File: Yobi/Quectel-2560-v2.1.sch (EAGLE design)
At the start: 110 parts, among them IC1 LM2576S, IC2 LM2576S, J1 U.FL, T1 NPN, T2 PNP, T3 NPN, U1 ATMEGA1280AU, U2 Quectel M95, U3 QUECTEL-L80

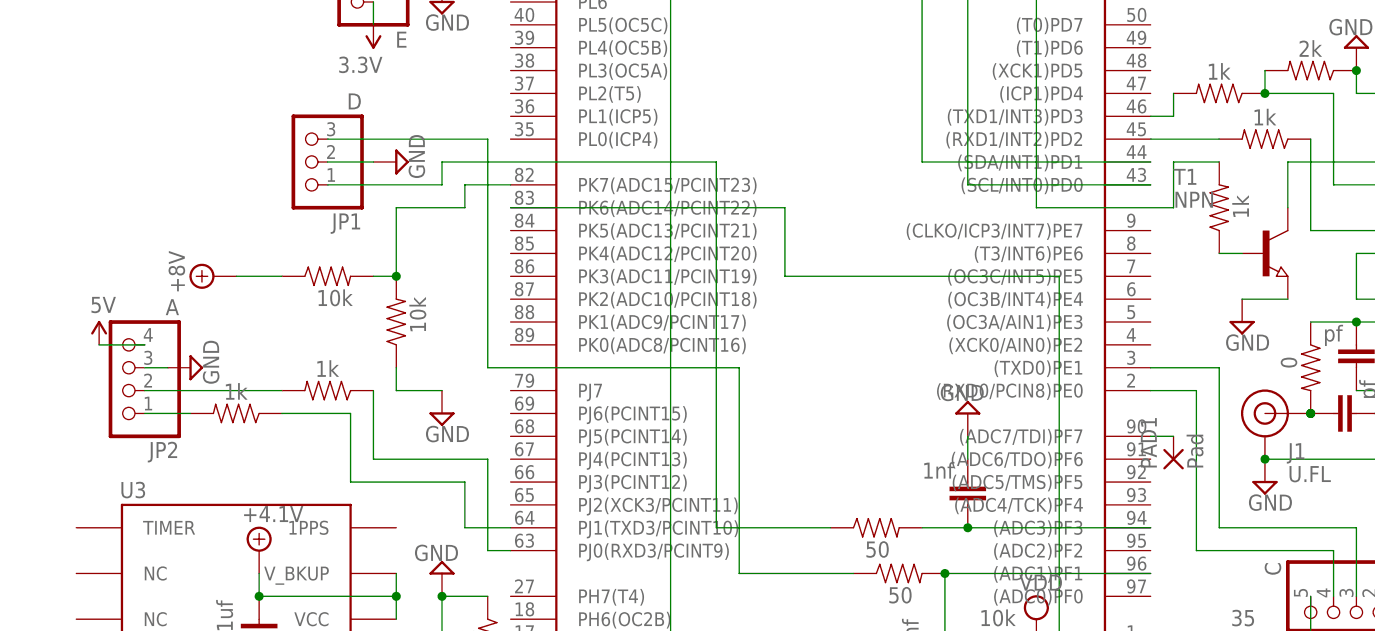
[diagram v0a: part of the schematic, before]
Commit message: cbdg
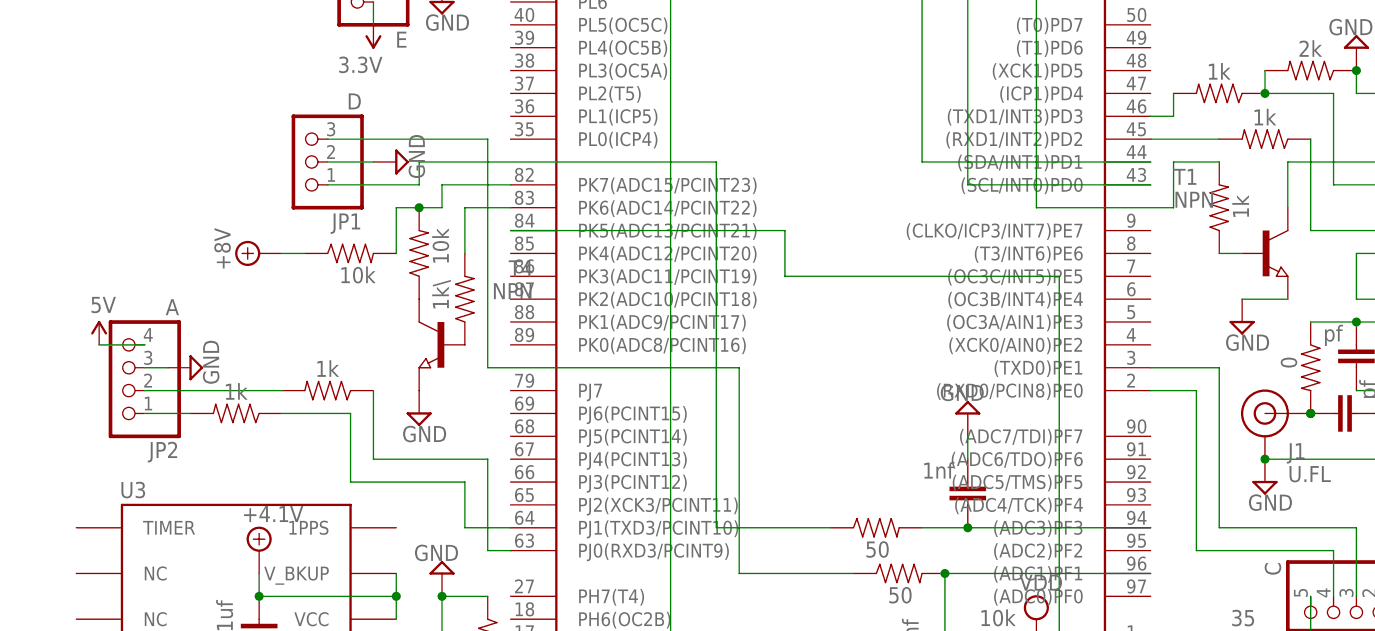
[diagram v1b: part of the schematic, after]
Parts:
- removed PAD1: Pad, wirepad:SMD2
- added R48: 1k\, SparkFun-Resistors:RESISTOR0805-RES
- added T4: NPN, semicon-smd-ipc:NPN-TRANSISTOR_SOT23
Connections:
- removed net N$69: PAD1.P, U1.(ADC7/TDI)PF7
- new net N$79: R44.1, T4.C
- new net N$80: R48.1, T4.B
- new net N$81: R48.2, U1.PK6(ADC14/PCINT22)
- net GND: now also T4.E; no longer R44.1
- net N$75: now also U1.PK5(ADC13/PCINT21); no longer U1.PK6(ADC14/PCINT22)
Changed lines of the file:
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@@
 <part name="DC16" library="resistor" deviceset="C-EU" device="C0805" value="0.1uf"/>
 <part name="JP11" library="pinhead" deviceset="PINHD-1X1" device="" value="Pogo Pin"/>
-<part name="PAD1" library="wirepad" deviceset="SMD2" device="" value="Pad"/>
 <part name="L4" library="rcl" deviceset="L-US" device="PIS2816" value="100uh"/>
 <part name="L2" library="rcl" deviceset="L-US" device="PIS2816" value="100uf"/>
+<part name="T4" library="semicon-smd-ipc" deviceset="NPN-TRANSISTOR_" device="SOT23" value="NPN"/>
+<part name="R48" library="SparkFun-Resistors" deviceset="RESISTOR" device="0805-RES" value="1k\"/>
 </parts>
 <sheets>
@@
 </instance>
 <instance part="SUPPLY54" gate="GND" x="104.14" y="71.12" rot="R270"/>
-<instance part="R43" gate="G$1" x="48.26" y="114.3" smashed="yes">
-<attribute name="VALUE" x="46.99" y="110.998" size="1.778" layer="96"/>
-</instance>
-<instance part="R44" gate="G$1" x="55.88" y="109.22" smashed="yes" rot="R90">
-<attribute name="VALUE" x="59.182" y="107.95" size="1.778" layer="96" rot="R90"/>
-</instance>
-<instance part="SUPPLY55" gate="+8V" x="35.56" y="114.3" rot="R90"/>
-<instance part="SUPPLY58" gate="GND" x="60.96" y="99.06"/>
+<instance part="R43" gate="G$1" x="50.8" y="116.84" smashed="yes">
+<attribute name="VALUE" x="49.53" y="113.538" size="1.778" layer="96"/>
+</instance>
+<instance part="R44" gate="G$1" x="58.42" y="116.84" smashed="yes" rot="R90">
+<attribute name="VALUE" x="61.722" y="115.57" size="1.778" layer="96" rot="R90"/>
+</instance>
+<instance part="SUPPLY55" gate="+8V" x="40.64" y="116.84" rot="R90"/>
+<instance part="SUPPLY58" gate="GND" x="58.42" y="99.06"/>
 <instance part="IC2" gate="A" x="142.24" y="292.1"/>
 <instance part="SUPPLY63" gate="+8V" x="119.38" y="297.18" rot="R90"/>
@@
 </instance>
 <instance part="JP11" gate="G$1" x="187.96" y="292.1"/>
-<instance part="PAD1" gate="1" x="142.24" y="93.98" rot="R90"/>
 <instance part="L4" gate="G$1" x="101.6" y="274.32" rot="R90"/>
 <instance part="L2" gate="G$1" x="165.1" y="292.1" rot="R90"/>
+<instance part="T4" gate="G$1" x="60.96" y="106.68" rot="MR0"/>
+<instance part="R48" gate="G$1" x="63.5" y="111.76" smashed="yes" rot="R90">
+<attribute name="VALUE" x="61.722" y="110.49" size="1.778" layer="96" rot="R90"/>
+</instance>
 </instances>
 <busses>
@@
 </segment>
 <segment>
+<pinref part="T4" gate="G$1" pin="E"/>
 <pinref part="SUPPLY58" gate="GND" pin="GND"/>
-<pinref part="R44" gate="G$1" pin="1"/>
-<wire x1="55.88" y1="104.14" x2="55.88" y2="101.6" width="0.1524" layer="91"/>
-<wire x1="55.88" y1="101.6" x2="60.96" y2="101.6" width="0.1524" layer="91"/>
 </segment>
 </net>
@@
 <segment>
 <pinref part="SUPPLY55" gate="+8V" pin="+8V"/>
-<wire x1="38.1" y1="114.3" x2="43.18" y2="114.3" width="0.1524" layer="91"/>
+<wire x1="43.18" y1="116.84" x2="45.72" y2="116.84" width="0.1524" layer="91"/>
 <pinref part="R43" gate="G$1" pin="1"/>
 </segment>
@@
 <wire x1="91.44" y1="86.36" x2="104.14" y2="86.36" width="0.1524" layer="91"/>
 <pinref part="R21" gate="G$1" pin="1"/>
-<wire x1="91.44" y1="127" x2="60.96" y2="127" width="0.1524" layer="91"/>
+<wire x1="91.44" y1="127" x2="58.42" y2="127" width="0.1524" layer="91"/>
 <pinref part="JP1" gate="A" pin="1"/>
-<wire x1="60.96" y1="127" x2="60.96" y2="124.46" width="0.1524" layer="91"/>
-<wire x1="60.96" y1="124.46" x2="48.26" y2="124.46" width="0.1524" layer="91"/>
+<wire x1="58.42" y1="127" x2="58.42" y2="124.46" width="0.1524" layer="91"/>
+<wire x1="58.42" y1="124.46" x2="48.26" y2="124.46" width="0.1524" layer="91"/>
 </segment>
 </net>
@@
 <wire x1="129.54" y1="71.12" x2="129.54" y2="114.3" width="0.1524" layer="91"/>
 <wire x1="129.54" y1="114.3" x2="99.06" y2="114.3" width="0.1524" layer="91"/>
-<pinref part="U1" gate="1" pin="PK6(ADC14/PCINT22)"/>
-<wire x1="99.06" y1="114.3" x2="99.06" y2="121.92" width="0.1524" layer="91"/>
-<wire x1="99.06" y1="121.92" x2="68.58" y2="121.92" width="0.1524" layer="91"/>
+<wire x1="99.06" y1="114.3" x2="99.06" y2="119.38" width="0.1524" layer="91"/>
+<pinref part="U1" gate="1" pin="PK5(ADC13/PCINT21)"/>
+<wire x1="68.58" y1="119.38" x2="99.06" y2="119.38" width="0.1524" layer="91"/>
 </segment>
 </net>
 <net name="N$76" class="0">
 <segment>
+<pinref part="R44" gate="G$1" pin="2"/>
+<wire x1="58.42" y1="121.92" x2="60.96" y2="121.92" width="0.1524" layer="91"/>
+<wire x1="60.96" y1="121.92" x2="60.96" y2="124.46" width="0.1524" layer="91"/>
+<pinref part="U1" gate="1" pin="PK7(ADC15/PCINT23)"/>
+<wire x1="60.96" y1="124.46" x2="68.58" y2="124.46" width="0.1524" layer="91"/>
 <pinref part="R43" gate="G$1" pin="2"/>
-<pinref part="R44" gate="G$1" pin="2"/>
-<wire x1="53.34" y1="114.3" x2="55.88" y2="114.3" width="0.1524" layer="91"/>
-<wire x1="55.88" y1="114.3" x2="55.88" y2="121.92" width="0.1524" layer="91"/>
-<wire x1="55.88" y1="121.92" x2="63.5" y2="121.92" width="0.1524" layer="91"/>
-<wire x1="63.5" y1="121.92" x2="63.5" y2="124.46" width="0.1524" layer="91"/>
-<pinref part="U1" gate="1" pin="PK7(ADC15/PCINT23)"/>
-<wire x1="63.5" y1="124.46" x2="68.58" y2="124.46" width="0.1524" layer="91"/>
-<junction x="55.88" y="114.3"/>
+<wire x1="58.42" y1="121.92" x2="55.88" y2="121.92" width="0.1524" layer="91"/>
+<wire x1="55.88" y1="121.92" x2="55.88" y2="116.84" width="0.1524" layer="91"/>
+<junction x="58.42" y="121.92"/>
 </segment>
 </net>
@@
 </segment>
 </net>
-<net name="N$69" class="0">
-<segment>
-<pinref part="PAD1" gate="1" pin="P"/>
-<pinref part="U1" gate="1" pin="(ADC7/TDI)PF7"/>
-<wire x1="142.24" y1="96.52" x2="139.7" y2="96.52" width="0.1524" layer="91"/>
-</segment>
-</net>
+<net name="N$79" class="0">
+<segment>
+<pinref part="R44" gate="G$1" pin="1"/>
+<pinref part="T4" gate="G$1" pin="C"/>
+</segment>
+</net>
+<net name="N$80" class="0">
+<segment>
+<pinref part="T4" gate="G$1" pin="B"/>
+<pinref part="R48" gate="G$1" pin="1"/>
+</segment>
+</net>
+<net name="N$81" class="0">
+<segment>
+<pinref part="R48" gate="G$1" pin="2"/>
+<wire x1="63.5" y1="116.84" x2="63.5" y2="121.92" width="0.1524" layer="91"/>
+<pinref part="U1" gate="1" pin="PK6(ADC14/PCINT22)"/>
+<wire x1="63.5" y1="121.92" x2="68.58" y2="121.92" width="0.1524" layer="91"/>
+</segment>
+</net>

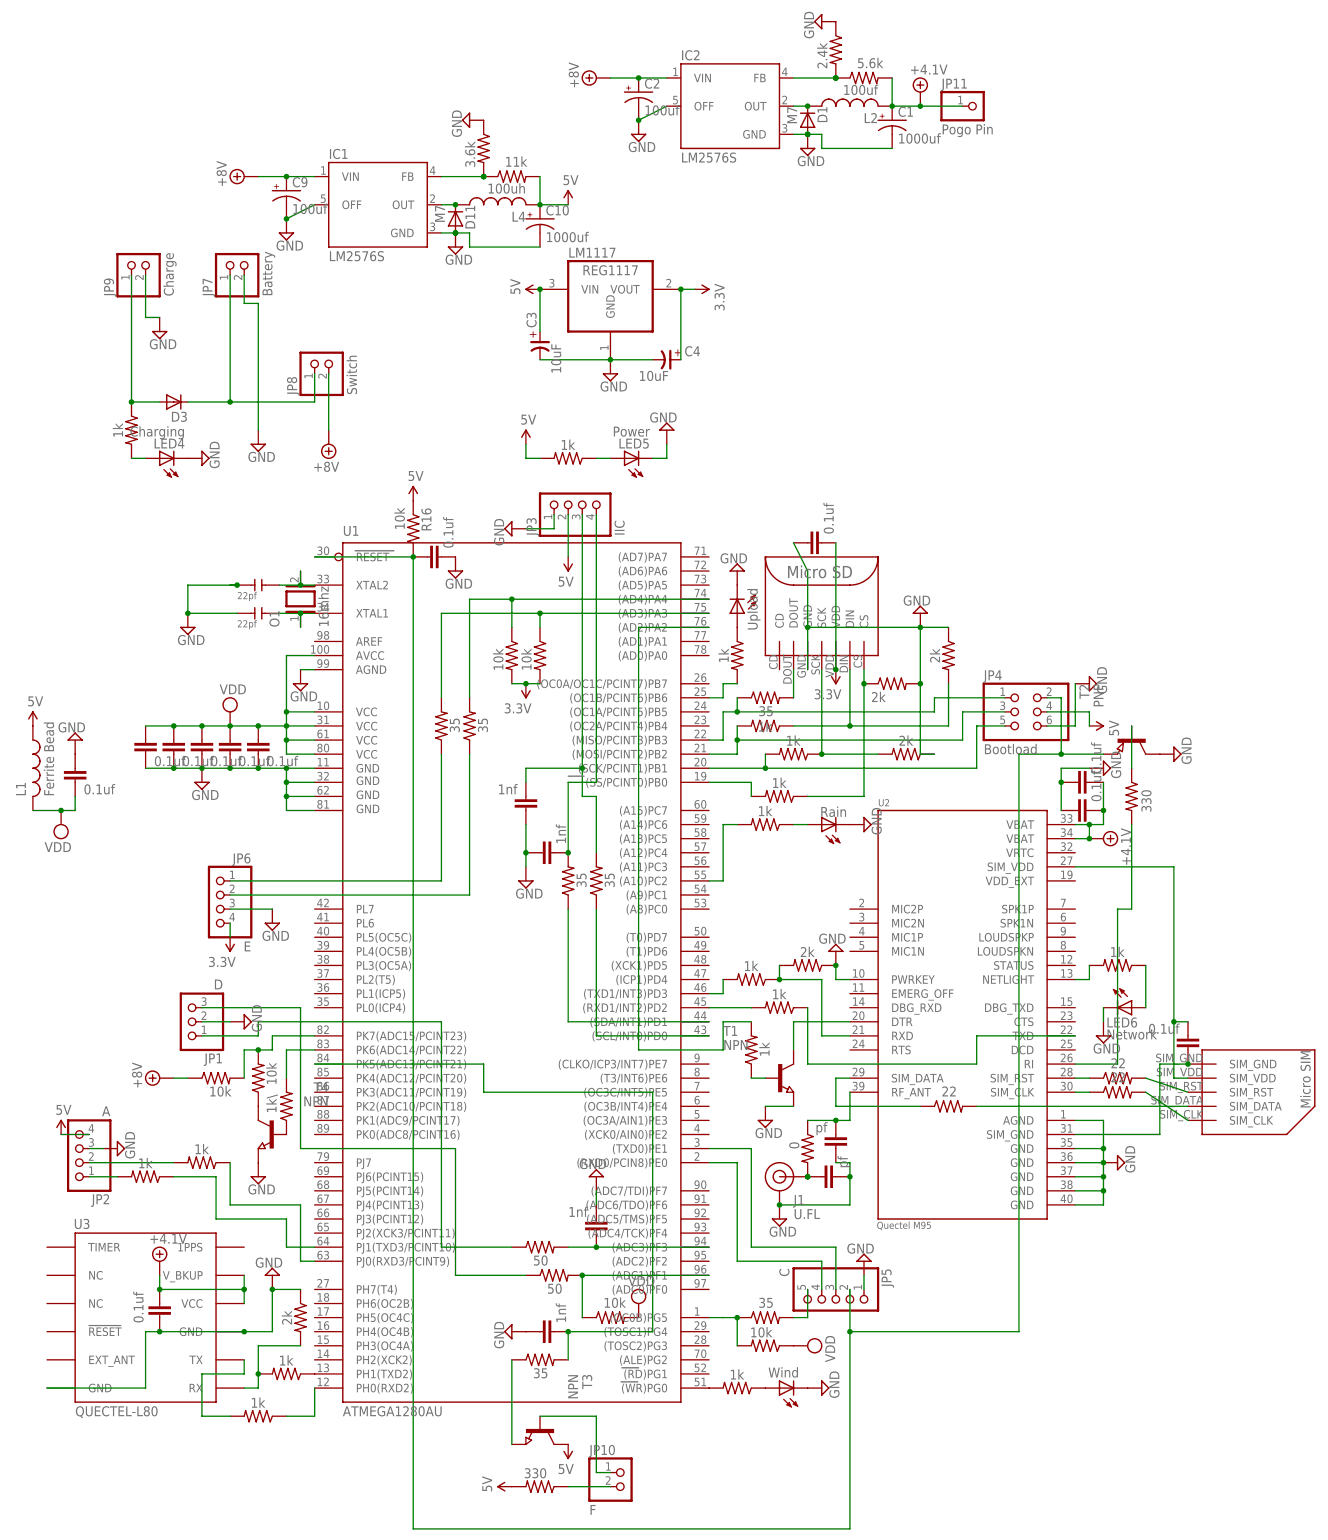
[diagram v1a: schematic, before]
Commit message: dfbfd
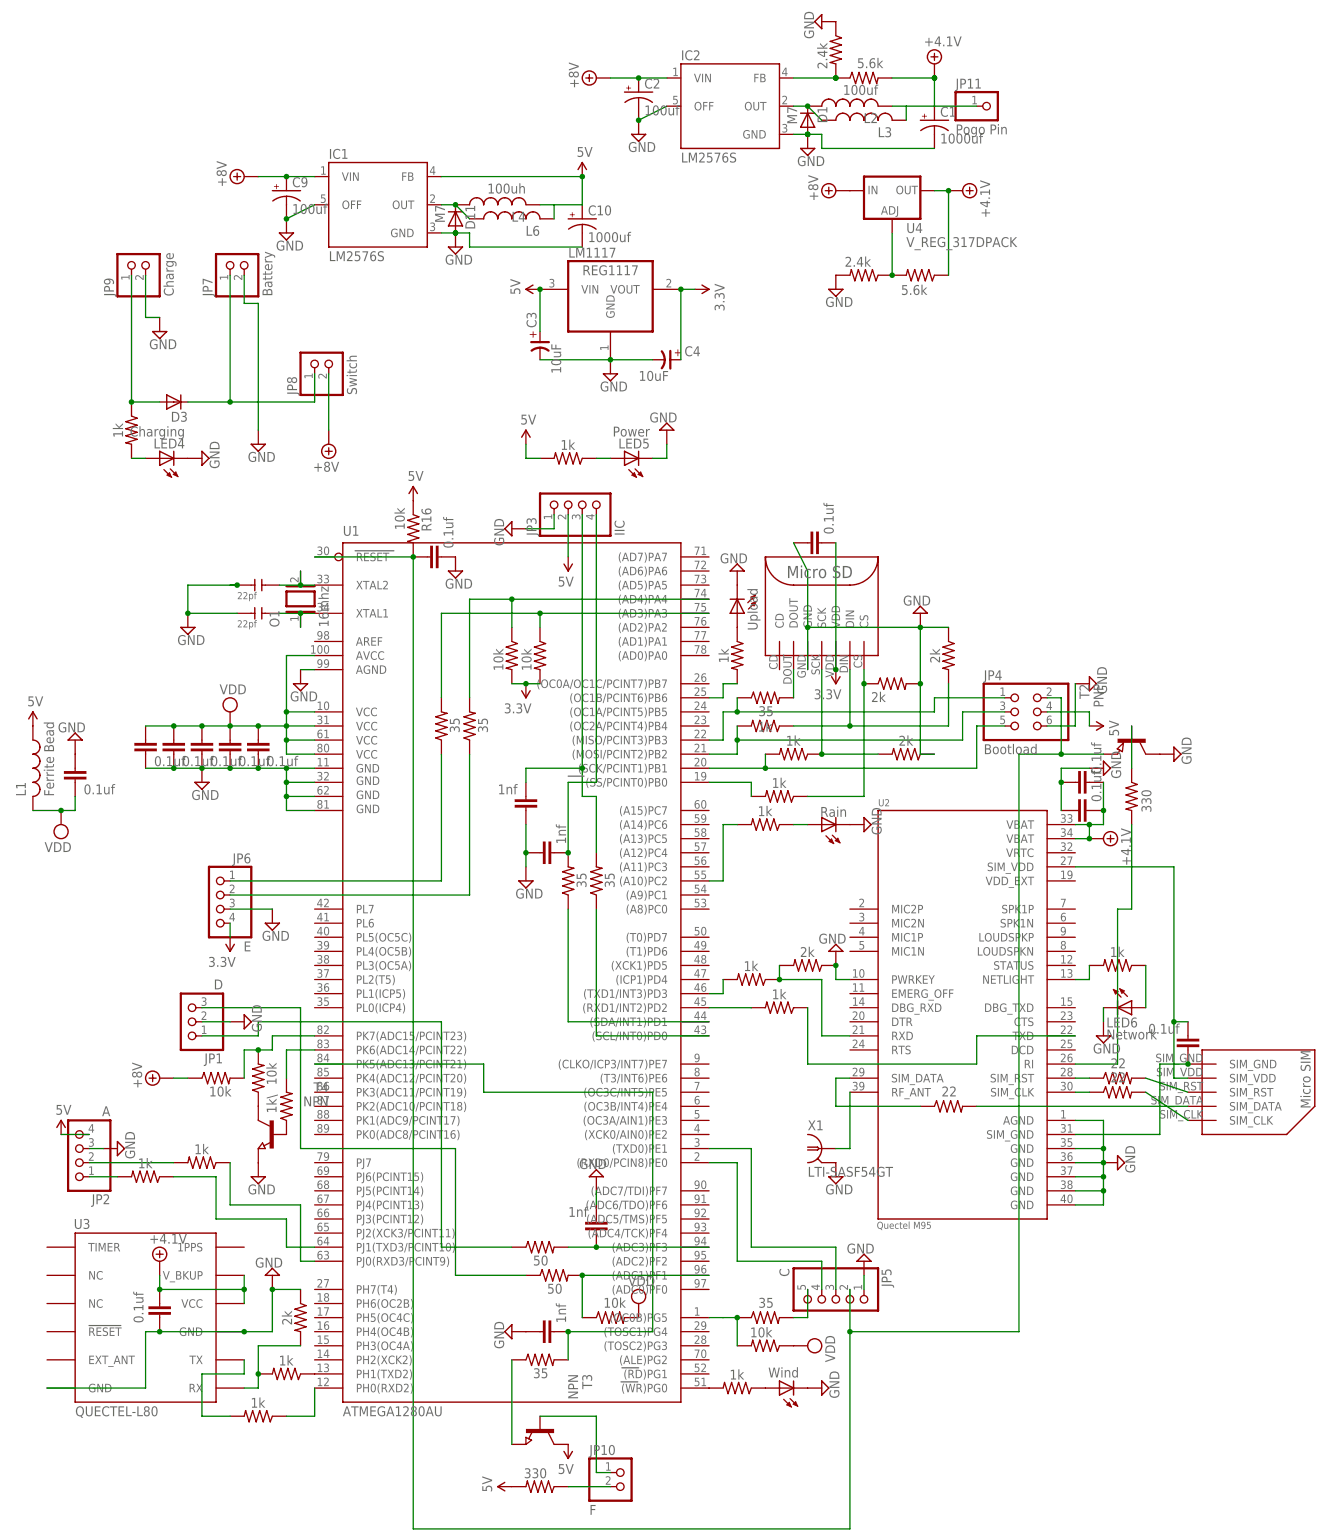
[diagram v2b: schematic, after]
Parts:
- removed DC8, DC9: pf, resistor:C-EUC0805
- removed J1: U.FL, SparkFun-Connectors:U.FL2PIN
- removed R1: 0, SparkFun-Resistors:RESISTOR0805-RES
- removed R2: 1k, SparkFun-Resistors:RESISTOR0805-RES
- removed R37: 3.6k, SparkFun-Resistors:RESISTOR0805-RES
- removed R38: 11k, SparkFun-Resistors:RESISTOR0805-RES
- removed T1: NPN, semicon-smd-ipc:NPN-TRANSISTOR_SOT23
- added L3, L6: (no value), rcl:L-US6000-XXX-RC
- added R49: 2.4k, SparkFun-Resistors:RESISTOR0805-RES
- added R50: 5.6k, SparkFun-Resistors:RESISTOR0805-RES
- added U4: V_REG_317DPACK, SparkFun-IC-Power:V_REG_317DPACK
- added X1: LTI-SASF54GT, con-coax:LTI-SASF54GT
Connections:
- removed net N$14: R2.2, U1.(AD2)PA2
- removed net N$15: R2.1, T1.B
- removed net N$46: T1.C, U2.DTR
- removed net N$5: DC9.1, J1.SIGNAL, R1.2
- removed net N$72: IC1.FB, R37.2, R38.1
- new net N$69: R49.1, R50.2, U4.ADJ
- net +4.1V: now also L3.2, R50.1, U4.OUT
- net +8V: now also U4.IN
- net 5V: now also IC1.FB, L6.2; no longer R38.2
- net GND: now also R49.2, X1.2; no longer DC8.1, DC9.2, J1.GND, R37.1, T1.E
- net N$21: now also X1.1; no longer DC8.2, R1.1
- net N$65: now also L6.1
- net N$77: now also L3.1
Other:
- moved on the sheet: C1, C10, JP11
